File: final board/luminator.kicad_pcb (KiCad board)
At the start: 2 copper layers, 6 parts

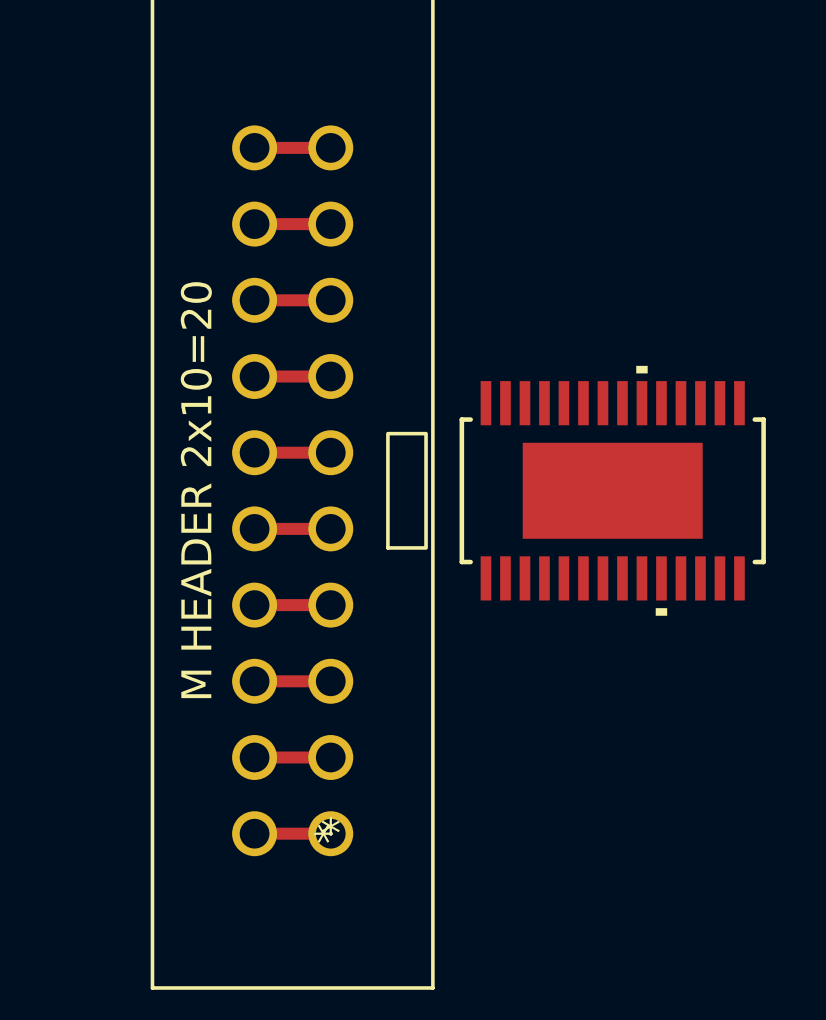
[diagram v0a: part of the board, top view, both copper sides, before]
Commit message: asd
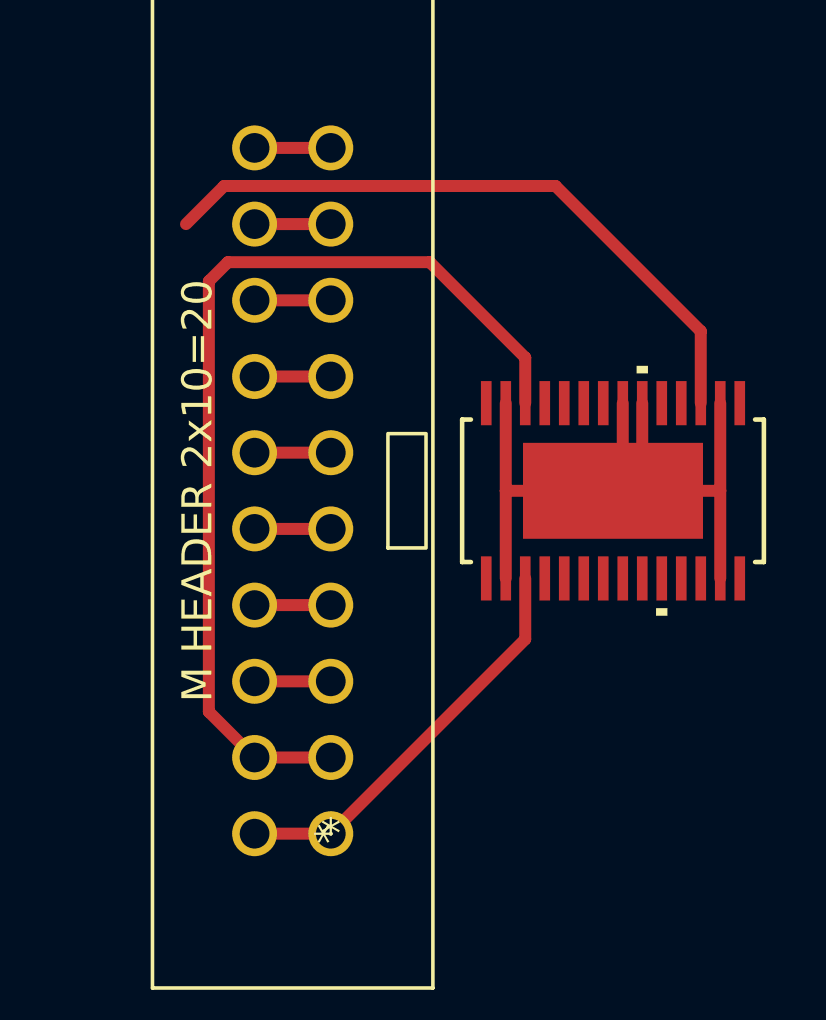
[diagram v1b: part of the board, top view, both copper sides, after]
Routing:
- net (no net): track 52.9 -> 141.6 mm
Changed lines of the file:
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@@
   )
   (footprint "Luminator:TSSOP-28EP_MPQ6628_MNP" (layer "F.Cu")
-    (at 111.252 119.888 90)
+    (at 111.261499 119.888 90)
     (tags "MPQ6628GF-AEC1-P ")
     (attr smd)
@@
     (effects (font (size 1 1) (thickness 0.15)))
   )
+  (segment (start 114.836498 119.888) (end 114.836498 122.809) (width 0.4) (layer "F.Cu") (net 0))
+  (segment (start 114.186499 114.567499) (end 109.347 109.728) (width 0.4) (layer "F.Cu") (net 0))
   (segment (start 99.314 126.238) (end 101.854 126.238) (width 0.4) (layer "F.Cu") (net 0))
   (segment (start 101.854 89.916) (end 100.584 88.646) (width 0.4) (layer "F.Cu") (net 0))
+  (segment (start 108.336499 124.835501) (end 108.336499 122.809) (width 0.4) (layer "F.Cu") (net 0))
+  (segment (start 107.6865 119.888) (end 107.6865 116.967) (width 0.4) (layer "F.Cu") (net 0))
   (segment (start 101.854 54.356) (end 101.854 51.816) (width 0.4) (layer "F.Cu") (net 0))
   (segment (start 99.314 110.998) (end 101.854 110.998) (width 0.4) (layer "F.Cu") (net 0))
@@
   (segment (start 101.854 123.698) (end 99.314 123.698) (width 0.4) (layer "F.Cu") (net 0))
   (segment (start 99.314 116.078) (end 101.854 116.078) (width 0.4) (layer "F.Cu") (net 0))
+  (segment (start 114.836498 116.967) (end 114.836498 119.888) (width 0.4) (layer "F.Cu") (net 0))
   (segment (start 101.854 56.896) (end 101.854 59.436) (width 0.4) (layer "F.Cu") (net 0))
+  (segment (start 109.347 109.728) (end 98.298 109.728) (width 0.4) (layer "F.Cu") (net 0))
   (segment (start 101.854 41.656) (end 100.584 42.926) (width 0.4) (layer "F.Cu") (net 0))
   (segment (start 101.854 113.538) (end 99.314 113.538) (width 0.4) (layer "F.Cu") (net 0))
+  (segment (start 97.79 112.903) (end 97.79 127.254) (width 0.4) (layer "F.Cu") (net 0))
   (segment (start 101.854 61.976) (end 101.854 64.516) (width 0.4) (layer "F.Cu") (net 0))
+  (segment (start 108.336499 116.967) (end 108.336499 115.448499) (width 0.4) (layer "F.Cu") (net 0))
+  (segment (start 111.5865 116.967) (end 111.5865 119.562999) (width 0.4) (layer "F.Cu") (net 0))
   (segment (start 101.854 77.216) (end 101.854 79.756) (width 0.4) (layer "F.Cu") (net 0))
   (segment (start 99.314 121.158) (end 101.854 121.158) (width 0.4) (layer "F.Cu") (net 0))
   (segment (start 101.854 128.778) (end 99.314 128.778) (width 0.4) (layer "F.Cu") (net 0))
+  (segment (start 105.156 112.268) (end 98.425 112.268) (width 0.4) (layer "F.Cu") (net 0))
   (segment (start 100.584 45.466) (end 101.854 46.736) (width 0.4) (layer "F.Cu") (net 0))
+  (segment (start 114.186499 116.967) (end 114.186499 114.567499) (width 0.4) (layer "F.Cu") (net 0))
+  (segment (start 108.336499 115.448499) (end 105.156 112.268) (width 0.4) (layer "F.Cu") (net 0))
   (segment (start 101.854 67.056) (end 101.854 69.596) (width 0.4) (layer "F.Cu") (net 0))
+  (segment (start 114.836498 119.888) (end 111.261499 119.888) (width 0.4) (layer "F.Cu") (net 0))
   (segment (start 100.584 42.926) (end 100.584 45.466) (width 0.4) (layer "F.Cu") (net 0))
   (segment (start 101.854 108.458) (end 99.314 108.458) (width 0.4) (layer "F.Cu") (net 0))
+  (segment (start 98.425 112.268) (end 97.79 112.903) (width 0.4) (layer "F.Cu") (net 0))
+  (segment (start 101.854 131.318) (end 108.336499 124.835501) (width 0.4) (layer "F.Cu") (net 0))
+  (segment (start 112.236498 118.913001) (end 111.261499 119.888) (width 0.4) (layer "F.Cu") (net 0))
   (segment (start 100.584 86.106) (end 101.854 84.836) (width 0.4) (layer "F.Cu") (net 0))
+  (segment (start 111.5865 119.562999) (end 111.261499 119.888) (width 0.4) (layer "F.Cu") (net 0))
   (segment (start 101.854 131.318) (end 99.314 131.318) (width 0.4) (layer "F.Cu") (net 0))
   (segment (start 100.584 88.646) (end 100.584 86.106) (width 0.4) (layer "F.Cu") (net 0))
   (segment (start 101.854 118.618) (end 99.314 118.618) (width 0.4) (layer "F.Cu") (net 0))
+  (segment (start 97.79 127.254) (end 99.314 128.778) (width 0.4) (layer "F.Cu") (net 0))
+  (segment (start 112.236498 116.967) (end 112.236498 118.913001) (width 0.4) (layer "F.Cu") (net 0))
+  (segment (start 98.298 109.728) (end 97.028 110.998) (width 0.4) (layer "F.Cu") (net 0))
+  (segment (start 107.6865 119.888) (end 111.261499 119.888) (width 0.4) (layer "F.Cu") (net 0))
+  (segment (start 107.6865 122.809) (end 107.6865 119.888) (width 0.4) (layer "F.Cu") (net 0))
 )
